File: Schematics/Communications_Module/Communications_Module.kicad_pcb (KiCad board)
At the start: 4 copper layers, 69.5 x 60 mm, 74 parts, among them J1 USB_C_Female_USB2_Small, J2 SWD_01x04_Pin, J3 Stack Male Edge Connector, Q1 AO3400A, SW1 SW_STM_RESET, SW2 SW_STM_BOOT_MODE, U1 RFM95W-915, U2 W25Q128JVS, U3 AMS1117-3.3, U4 LM66100DCKR, U5 LM66100DCKR, U6 LM66100DCKR, U7 STM32F103CBT6, U8 ACS70331EOLC, U9 ISO1042BDWVR, Y1 X322516MMB4SI

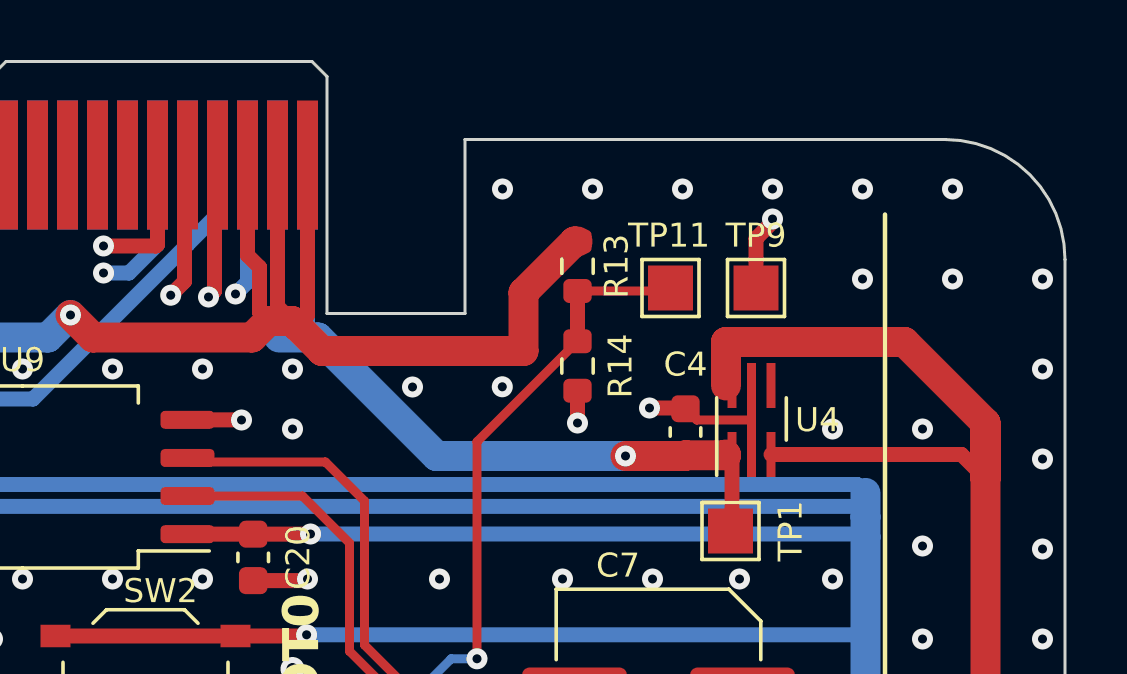
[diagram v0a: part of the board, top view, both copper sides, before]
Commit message: Very minor PCB tweaks
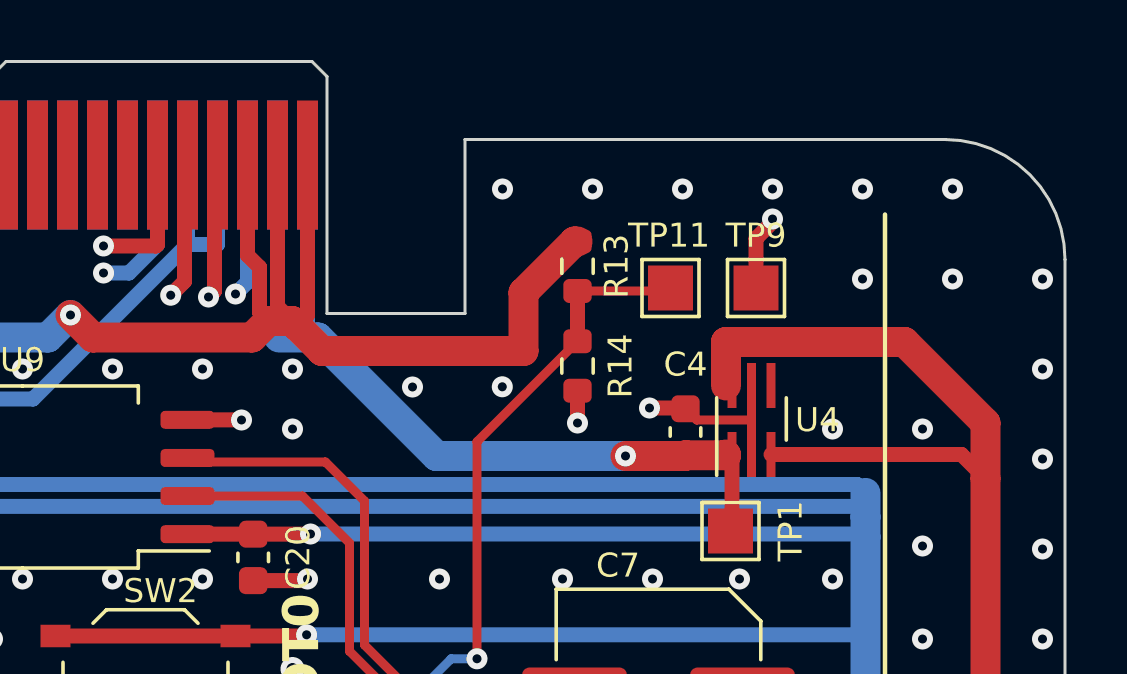
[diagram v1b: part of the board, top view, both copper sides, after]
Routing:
- net V_MUX: track 127.0 -> 125.1 mm
- net +5V: track 31.8 -> 32.4 mm
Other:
- board text removed: "-->"
- board text removed: "IDK what to do about these ground pins"
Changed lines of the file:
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@@
-    (effects (font (size 1 1) (thickness 0.15)) (justify left bottom))
-  )
-  (gr_text "-->" (at 143.9 70.6 -90) (layer "Cmts.User")
     (effects (font (size 1 1) (thickness 0.15)) (justify left bottom))
   )
   (gr_text "USE GRID THAT IS SOME\nMULTIPLE OF 0.1mm\n\n(0.1mm, 0.2mm, 0.5mm, 1.0mm, etc)" (at 177.6 133.2) (layer "Cmts.User")
-    (effects (font (size 1 1) (thickness 0.15)) (justify left bottom))
-  )
-  (gr_text "IDK what to do about these ground pins" (at 132.3 70.5) (layer "Cmts.User")
     (effects (font (size 1 1) (thickness 0.15)) (justify left bottom))
   )
@@
   (segment (start 133.495 92.76) (end 133.495 90.51) (width 0.5) (layer "F.Cu") (net 3))
   (via (at 130.725 86.027707) (size 0.7) (drill 0.3) (layers "F.Cu" "B.Cu") (net 3))
-  (segment (start 145.5 79.85) (end 144.5 80.85) (width 0.5) (layer "B.Cu") (net 3))
-  (segment (start 145.5 78.2) (end 145.5 79.85) (width 0.5) (layer "B.Cu") (net 3))
   (segment (start 139.35 86) (end 130.752707 86) (width 0.5) (layer "B.Cu") (net 3))
+  (segment (start 145.5 78.2) (end 145.5 80.85) (width 0.5) (layer "B.Cu") (net 3))
   (segment (start 144.5 80.85) (end 139.35 86) (width 0.5) (layer "B.Cu") (net 3))
+  (segment (start 145.5 80.85) (end 144.5 80.85) (width 0.5) (layer "B.Cu") (net 3))
   (segment (start 144.5 78.2) (end 144.5 80.85) (width 0.5) (layer "B.Cu") (net 3))
   (segment (start 130.752707 86) (end 130.725 86.027707) (width 0.5) (layer "B.Cu") (net 3))
@@
   (segment (start 171.05 95.75) (end 171.1 95.8) (width 1) (layer "F.Cu") (net 27))
   (segment (start 169.5 118.2) (end 171.1 116.6) (width 0.5) (layer "F.Cu") (net 27))
-  (segment (start 171.1 88.65) (end 171.1 86.8) (width 1) (layer "F.Cu") (net 27))
   (segment (start 163.05 106.5) (end 163.7 105.85) (width 0.5) (layer "F.Cu") (net 27))
   (segment (start 168.4 84.1) (end 162.45 84.1) (width 1) (layer "F.Cu") (net 27))
